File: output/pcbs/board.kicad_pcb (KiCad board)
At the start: 2 copper layers, 140.2 x 108.1 mm, 41 parts

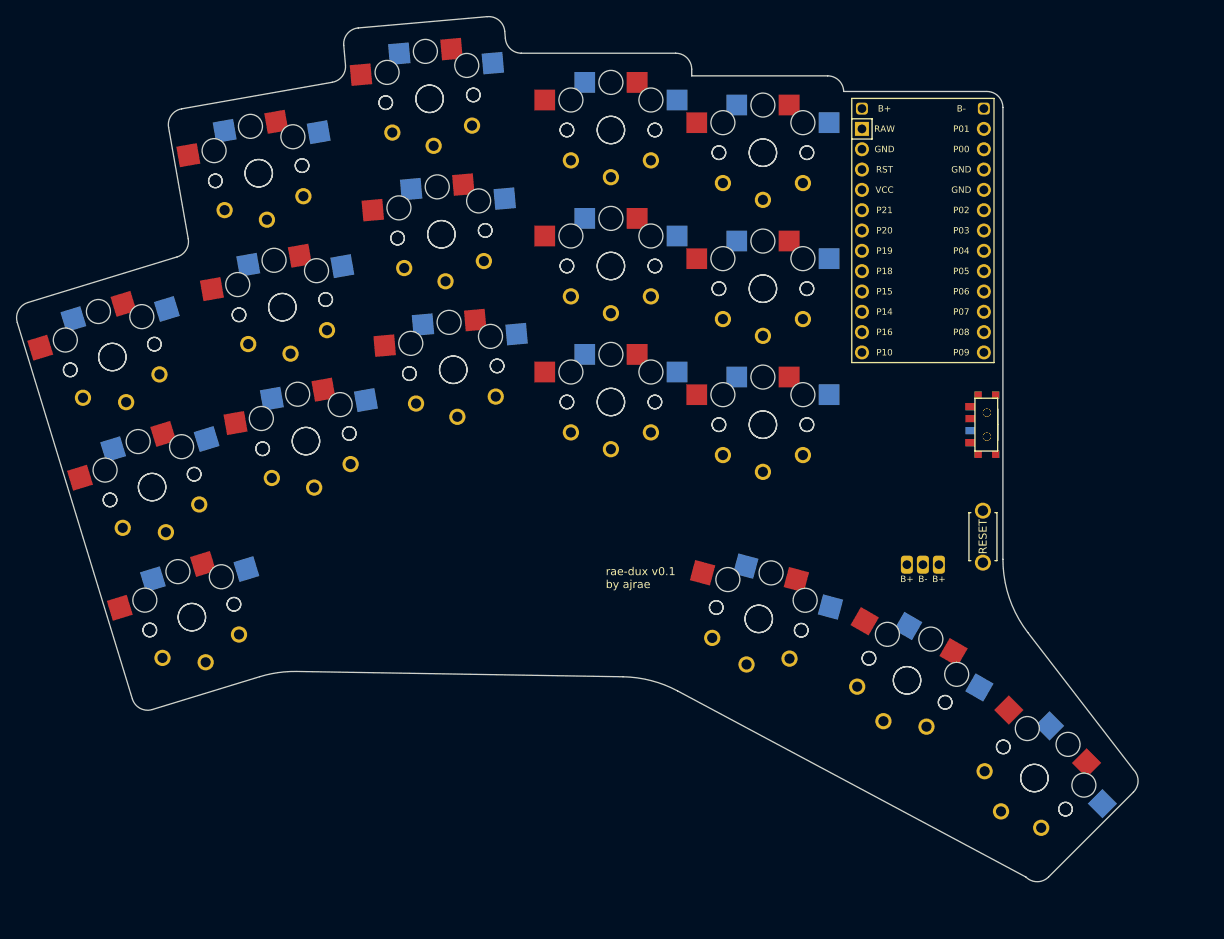
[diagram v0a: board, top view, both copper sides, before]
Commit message: add latest output
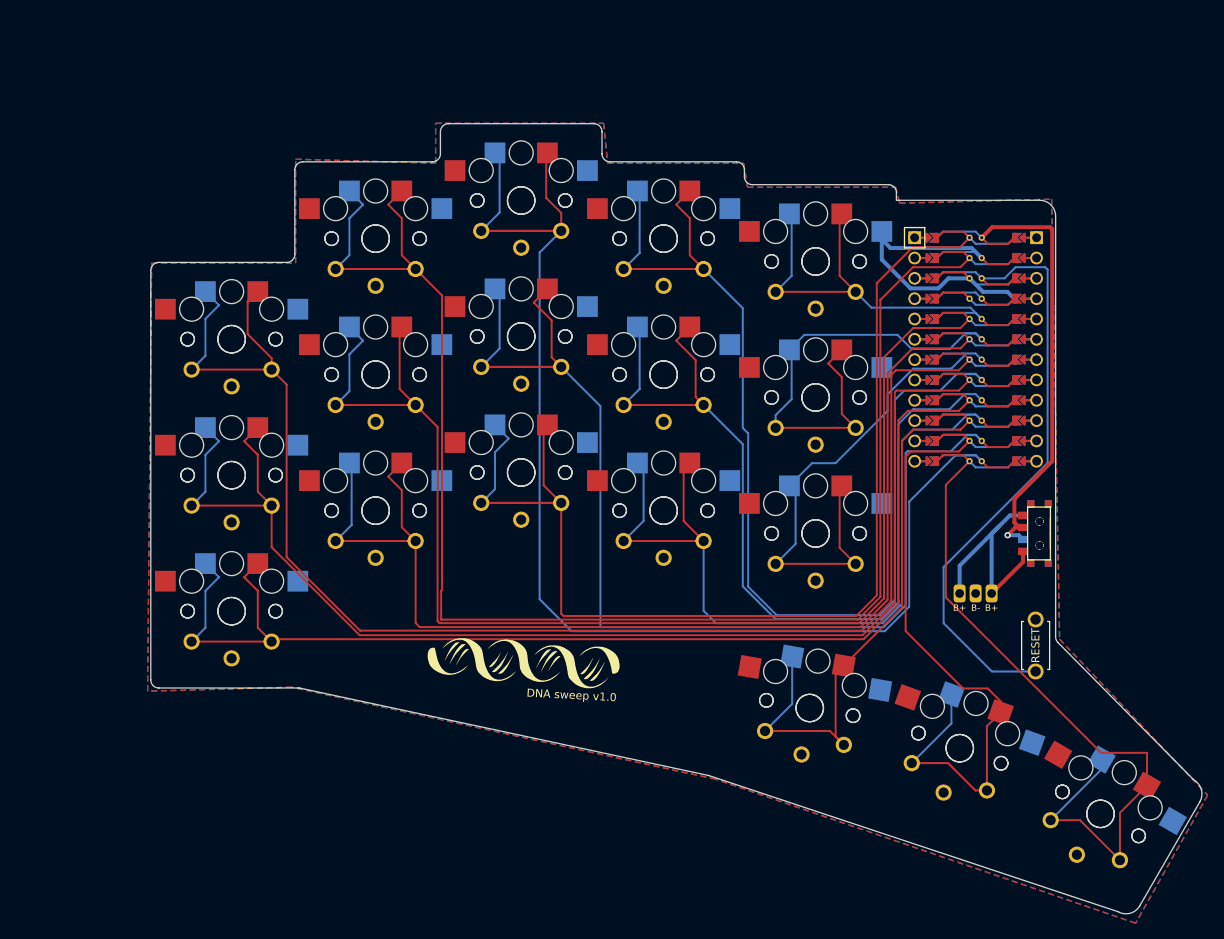
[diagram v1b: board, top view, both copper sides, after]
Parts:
- added G***: LOGO, LOGO, F.Cu at (104.5, -43.5)
- added G***: LOGO, LOGO, B.Cu at (104.5, -44.0)
- moved S17 17.1 mm to (104.2, -101.3), turned to 0 degrees
- moved S18 17.1 mm to (104.2, -101.3), turned to 180 degrees
- moved S11 16.7 mm to (86.0, -96.6), turned to 0 degrees
- moved S12 16.7 mm to (86.0, -96.6), turned to 180 degrees
- moved S15 16.2 mm to (104.2, -84.3), turned to 0 degrees
- moved S16 16.2 mm to (104.2, -84.3), turned to 180 degrees
- moved S13 15.4 mm to (104.2, -67.3), turned to 0 degrees
- moved S14 15.4 mm to (104.2, -67.3), turned to 180 degrees
- moved S27 15.1 mm to (141.0, -76.7)
- moved S28 15.1 mm to (141.0, -76.7)
- moved MCU1 15.1 mm to (161.0, -82.7)
- moved S29 15.1 mm to (141.0, -93.7)
- moved S30 15.1 mm to (141.0, -93.7)
- moved B1 15.1 mm to (168.5, -45.7)
- moved S25 15.1 mm to (141.0, -59.7)
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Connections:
- MCU1 pad 13: P1 -> P9
- MCU1 pad 14: P0 -> P8
- MCU1 pad 15: GND -> P7
- MCU1 pad 16: GND -> P6
- MCU1 pad 17: P2 -> P5
- MCU1 pad 18: P3 -> P4
- MCU1 pad 19: P4 -> P3
- MCU1 pad 20: P5 -> P2
- MCU1 pad 21: P6 -> GND
- MCU1 pad 22: P7 -> GND
- MCU1 pad 23: P8 -> P0
- MCU1 pad 24: P9 -> P1
- S15 pad 1: P18 -> P16
- S16 pad 1: P18 -> P16
- S17 pad 1: P15 -> P10
- S18 pad 1: P15 -> P10
- S21 pad 1: P16 -> P15
- S22 pad 1: P16 -> P15
- S23 pad 1: P10 -> P18
- S24 pad 1: P10 -> P18
- T1 pad 2: Bplus -> RAW
- T2 pad 2: Bplus -> RAW
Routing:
- net P0: track 0.00 -> 185.5 mm
- net P4: track 0.00 -> 177.4 mm
- net P2: track 0.00 -> 160.7 mm
- net P5: track 0.00 -> 159.4 mm
- net P10: track 0.00 -> 152.7 mm
- net P6: track 0.00 -> 147.5 mm
- net P3: track 0.00 -> 143.8 mm
- net P1: track 0.00 -> 140.2 mm
- net P16: track 0.00 -> 136.4 mm
- net P18: track 0.00 -> 132.7 mm
- net P15: track 0.00 -> 111.2 mm
- net P14: track 0.00 -> 99.4 mm
- net P9: track 0.00 -> 87.2 mm
- net P8: track 0.00 -> 79.4 mm
- net P7: track 0.00 -> 72.6 mm
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- added copper zone on B.Cu, net GND
- added copper zone on F.Cu, net GND
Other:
- board size 140.2 x 108.1 mm -> 131.4 x 98.8 mm
- net class Default removed
- net class Power removed
- board text added: "DNA sweep v1.0"
- board text removed: "rae-dux v0.1 by ajrae"
